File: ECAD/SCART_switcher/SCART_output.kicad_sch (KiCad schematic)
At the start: 10 parts, among them J2 RCA Left, J3 RCA Right, Q3 BC847

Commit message: Progressed ECAD.
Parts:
- Q3: MFN BC847B,215 -> (none); MPN (none) -> BC847B,215
- R7, R?: MPN (none) -> RC0805FR-0710KL
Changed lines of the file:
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@@
       (effects (font (size 1.27 1.27)) hide)
     )
-    (property "Datasheet" "~" (at 105.41 77.47 0)
+    (property "Datasheet" "https://datasheet.lcsc.com/lcsc/1810201611_YAGEO-RC0805FR-0710KL_C84376.pdf" (at 105.41 77.47 0)
+      (effects (font (size 1.27 1.27)) hide)
+    )
+    (property "MPN" "RC0805FR-0710KL" (at 105.41 77.47 0)
       (effects (font (size 1.27 1.27)) hide)
     )
@@
     )
     (property "Datasheet" " ~" (at 220.98 123.19 0)
-      (effects (font (size 1.27 1.27)) hide)
-    )
-    (property "MFN" "" (at 220.98 124.46 0)
       (effects (font (size 1.27 1.27)) hide)
     )
@@
       (effects (font (size 1.27 1.27)) hide)
     )
-    (property "Datasheet" "~" (at 81.28 64.77 0)
-      (effects (font (size 1.27 1.27)) hide)
-    )
-    (property "MFN" "" (at 81.28 64.77 0)
+    (property "Datasheet" "https://datasheet.lcsc.com/lcsc/1810201611_YAGEO-RC0805FR-0710KL_C84376.pdf" (at 81.28 64.77 0)
+      (effects (font (size 1.27 1.27)) hide)
+    )
+    (property "MPN" "RC0805FR-0710KL" (at 81.28 64.77 0)
       (effects (font (size 1.27 1.27)) hide)
     )
@@
       (effects (font (size 1.27 1.27)) (justify left) hide)
     )
-    (property "MFN" "BC847B,215" (at 78.74 73.66 0)
-      (effects (font (size 1.27 1.27)) hide)
-    )
+    (property "MPN" "BC847B,215" (at 78.74 73.66 0)
+      (effects (font (size 1.27 1.27)) hide)
+    )

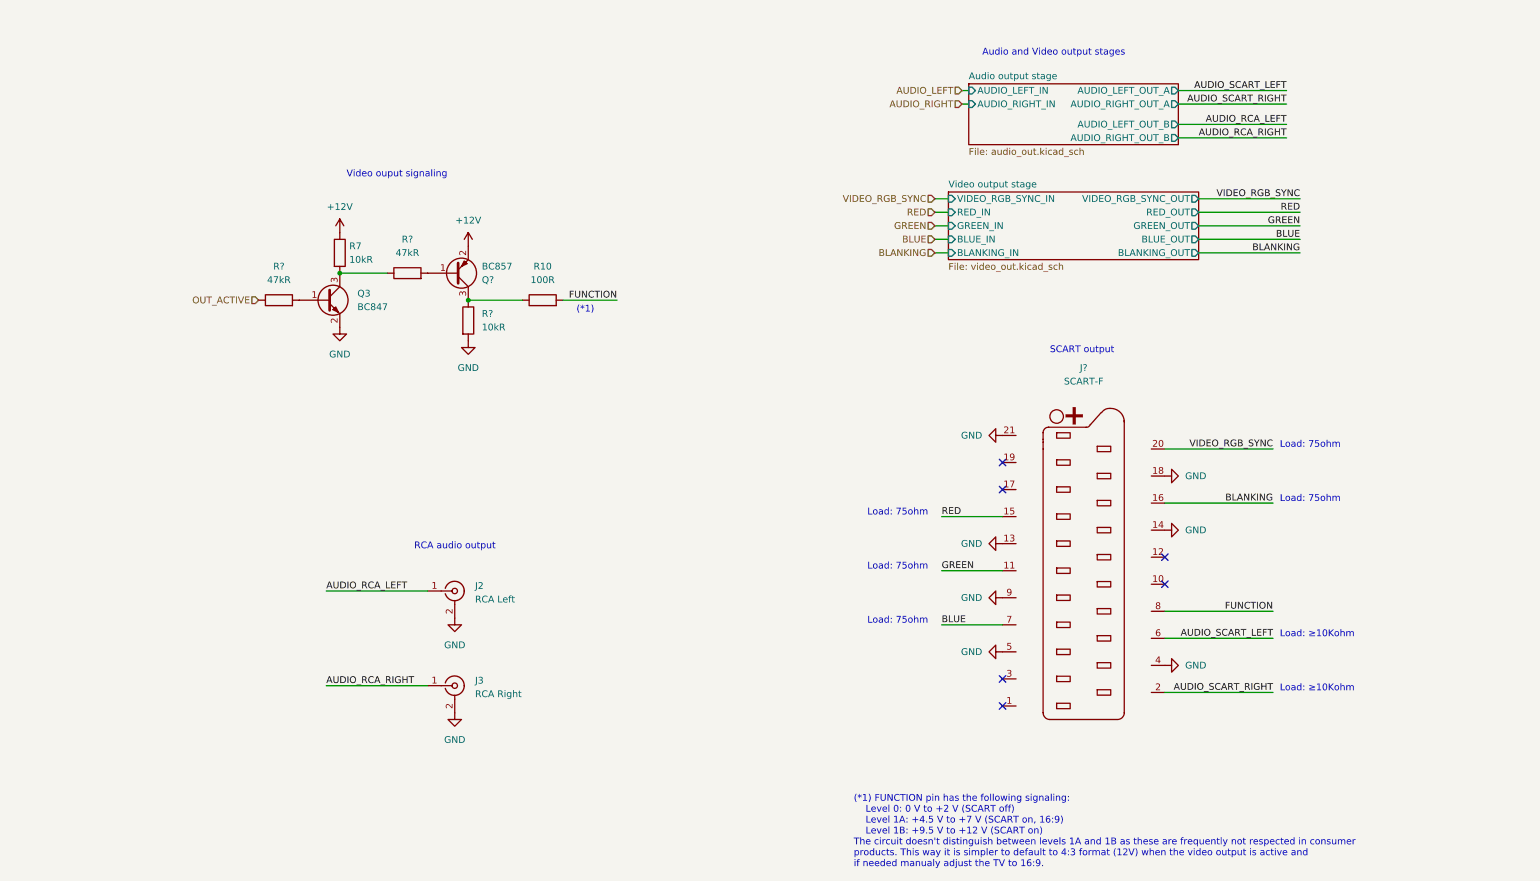
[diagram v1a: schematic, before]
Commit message: Progressed ECAD.
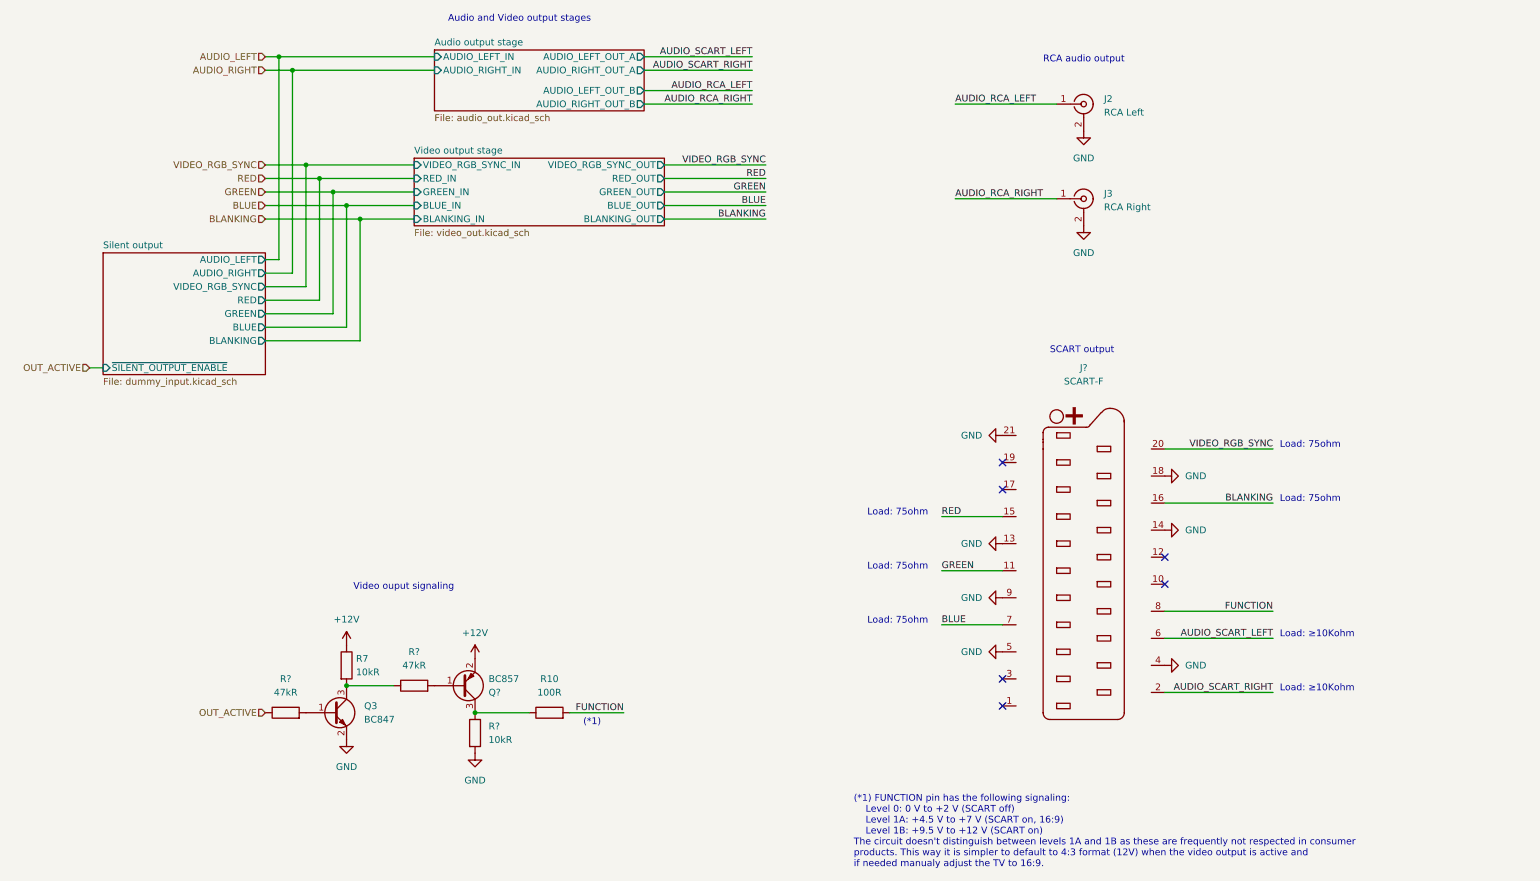
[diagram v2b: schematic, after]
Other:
- added sheet Silent output (dummy_input.kicad_sch)
- moved on the sheet: J2, J3, Q3, Q?, R10, R7, R?
